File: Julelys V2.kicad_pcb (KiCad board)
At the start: 2 copper layers, 73 x 89 mm, 38 parts, among them J1 USB_B_Micro, J2 Conn_01x04_Pin, J3 Conn_01x14_Pin, SW1 SW_Push, SW2 SW_Push, U1 ESP32-C3-WROOM-02, U2 74HC4051, U3 AMS1117-3.3

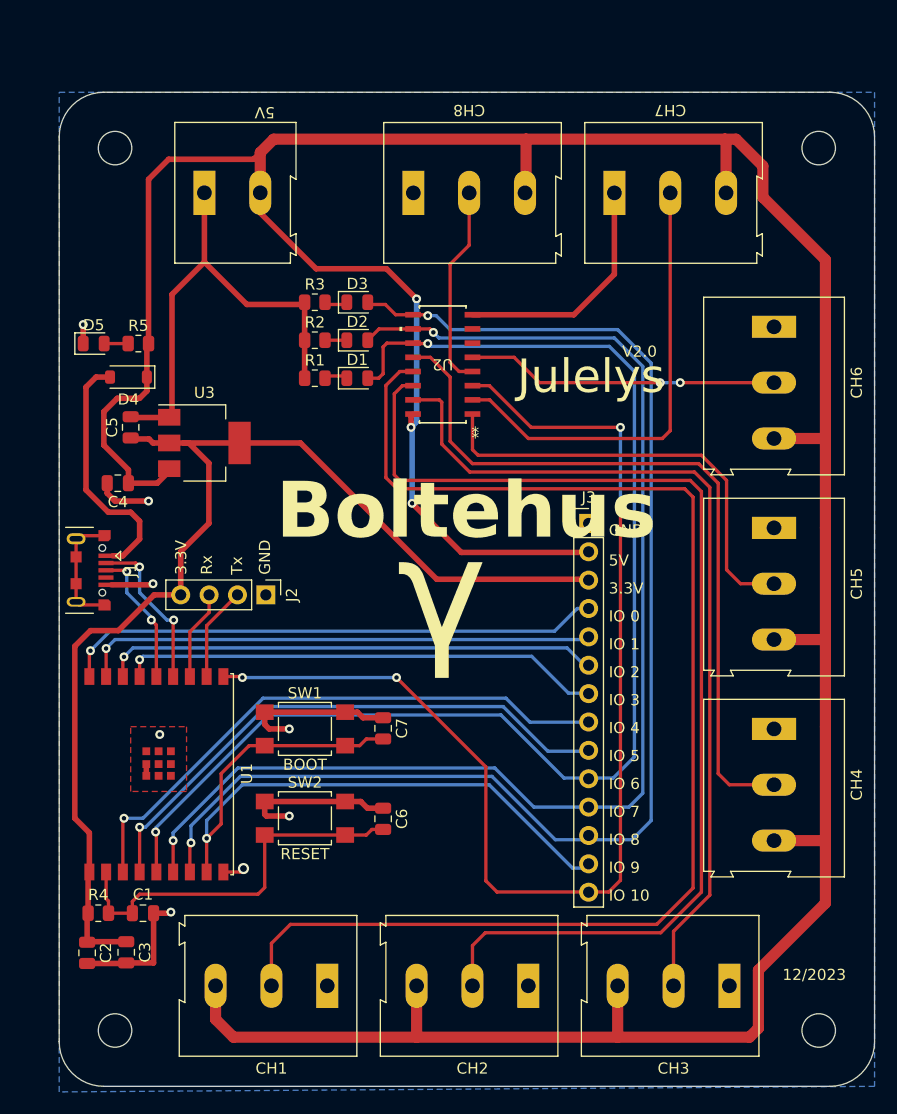
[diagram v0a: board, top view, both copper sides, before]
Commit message: version 3
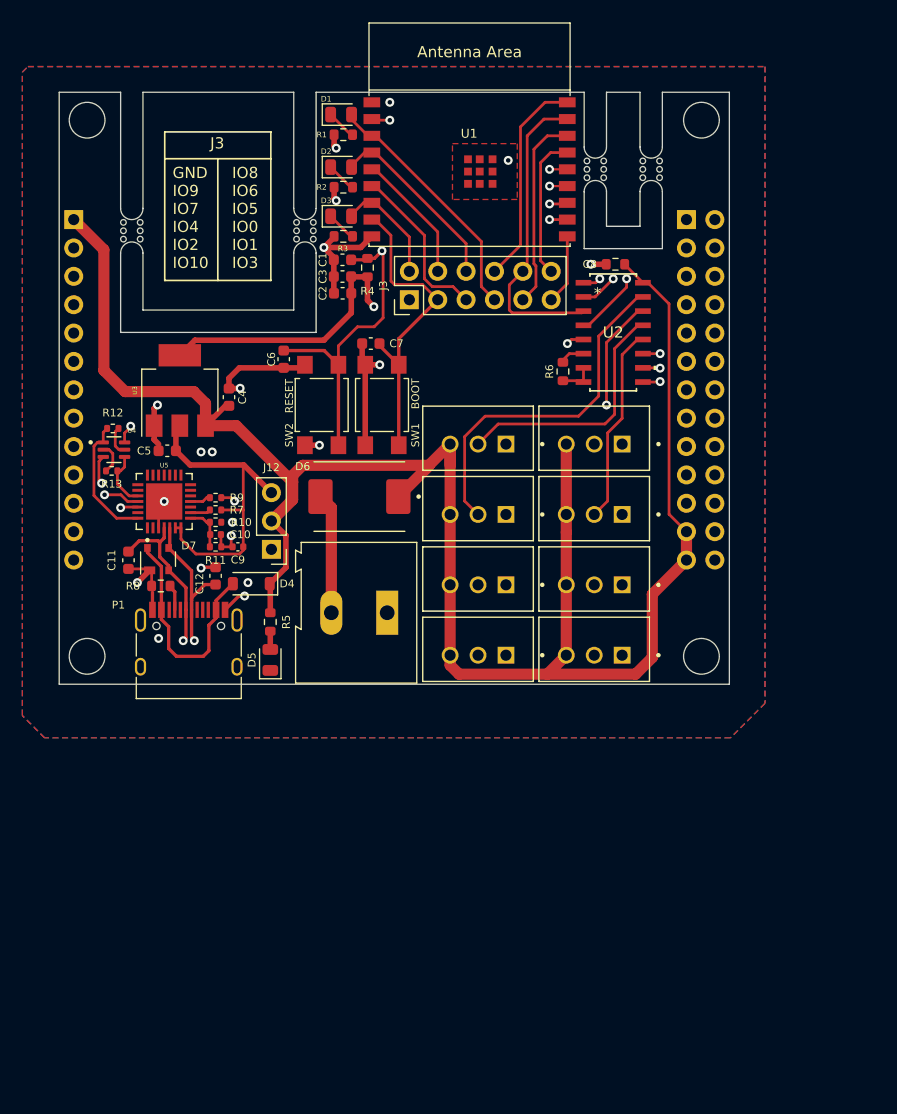
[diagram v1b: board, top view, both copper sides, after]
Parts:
- removed CH1, CH2, CH3, CH4, CH5, CH6, CH7, CH8: Screw_Terminal_01x03, TerminalBlock:TerminalBlock_Altech_AK300-3_P5.00mm
- added C10: 1uF/16V(10%), Capacitor_SMD:C_0402_1005Metric, F.Cu at (40.0, 54.6)
- added C11: 22pf, Capacitor_SMD:C_0603_1608Metric, F.Cu at (32.2, 56.9)
- added C12: 22pf, Capacitor_SMD:C_0603_1608Metric, F.Cu at (40.0, 58.3)
- added C8: 100nf, Resistor_SMD:R_0603_1608Metric, F.Cu at (75.8, 30.4)
- added C9: 10uF/25V(20%), Capacitor_SMD:C_0402_1005Metric, F.Cu at (42.0, 55.7)
- added D6: SS34-E3_57T, Diode_SMD:DIOM7959X262N, F.Cu at (52.9, 51.2)
- added D7: SP0503BAHT, Package_TO_SOT_SMD:SOT-143, F.Cu at (34.9, 56.8)
- added J10: B3B-XH-A, Connector:JST_B3B-XH-A, F.Cu at (63.5, 64.9)
- added J11: B3B-XH-A, Connector:JST_B3B-XH-A, F.Cu at (73.9, 64.9)
- added J12: Conn_01x03_Pin, Connector_PinHeader_2.54mm:PinHeader_1x03_P2.54mm_Vertical, F.Cu at (45.0, 55.9)
- added J4: B3B-XH-A, Connector:JST_B3B-XH-A, F.Cu at (63.5, 46.0)
- added J5: B3B-XH-A, Connector:JST_B3B-XH-A, F.Cu at (73.9, 46.0)
- added J6: B3B-XH-A, Connector:JST_B3B-XH-A, F.Cu at (63.5, 52.3)
- added J7: B3B-XH-A, Connector:JST_B3B-XH-A, F.Cu at (73.9, 52.3)
- added J8: B3B-XH-A, Connector:JST_B3B-XH-A, F.Cu at (63.5, 58.6)
- added J9: B3B-XH-A, Connector:JST_B3B-XH-A, F.Cu at (73.9, 58.6)
- added P1: USB_C_Plug_USB2.0, Connector_USB:USB_C_Receptacle_HRO_TYPE-C-31-M-12, F.Cu at (37.6, 65.4)
- added R10: 22.1K, Resistor_SMD:R_0402_1005Metric, F.Cu at (40.0, 53.5)
- added R11: 47.5K, Resistor_SMD:R_0402_1005Metric, F.Cu at (40.0, 55.7)
- added R12: 10k, Resistor_SMD:R_0402_1005Metric, F.Cu at (30.8, 45.1)
- added R13: 10k, Resistor_SMD:R_0402_1005Metric, F.Cu at (30.7, 48.9)
- added R6: 10K, Resistor_SMD:R_0603_1608Metric, F.Cu at (71.1, 40.0)
- added R7: 1K, Resistor_SMD:R_0402_1005Metric, F.Cu at (40.0, 52.4)
- added R8: 5.1K, Resistor_SMD:R_0603_1608Metric, F.Cu at (35.1, 59.2)
- added R9: 10K, Resistor_SMD:R_0402_1005Metric, F.Cu at (40.0, 51.3)
- added U4: BC847BDW1T1G, Transistor_Power_Module:SOT65P210X110-6N, F.Cu at (30.9, 47.0)
- added U5: CP2102N-A02-GQFN28, Connector_USB:QFN50P500X500X80-29N, F.Cu at (35.4, 51.6)
- added mouse-bite-2mm-slot: VAL**, footprints:mouse-bite-2mm-slot, F.Cu at (74.0, 21.9)
- added mouse-bite-2mm-slot: VAL**, footprints:mouse-bite-2mm-slot, F.Cu at (32.5, 27.4)
- added mouse-bite-2mm-slot: VAL**, footprints:mouse-bite-2mm-slot, F.Cu at (79.0, 21.9)
- added mouse-bite-2mm-slot: VAL**, footprints:mouse-bite-2mm-slot, F.Cu at (48.0, 27.4)
- C1, C2, C3, C4, C5, C6, C7: footprint Capacitor_SMD:C_0805_2012Metric -> Capacitor_SMD:C_0603_1608Metric
- H1, H2, H3, H4: footprint MountingHole:MountingHole_3mm -> MountingHole:MountingHole_3.2mm_M3
- J1: value USB_B_Micro -> Conn_02x13_Top_Bottom; footprint Connector_USB:USB_Micro-B_XKB_U254-051T-4BH83-F1S -> Connector_PinSocket_2.54mm:PinSocket_2x13_P2.54mm_Vertical; moved to B.Cu
- J2: value Conn_01x04_Pin -> Conn_01x13; footprint Connector_PinHeader_2.54mm:PinHeader_1x04_P2.54mm_Vertical -> Connector_PinSocket_2.54mm:PinSocket_1x13_P2.54mm_Vertical; moved to B.Cu
- J3: value Conn_01x14_Pin -> Conn_02x06_Odd_Even; footprint Connector_PinHeader_2.54mm:PinHeader_1x14_P2.54mm_Vertical -> Connector_PinHeader_2.54mm:PinHeader_2x06_P2.54mm_Vertical
- R1, R2, R3, R4, R5: footprint Resistor_SMD:R_0805_2012Metric -> Resistor_SMD:R_0603_1608Metric
- moved C3 63.5 mm to (51.4, 31.5), turned to 180 degrees
- moved C2 63.3 mm to (51.4, 33.0), turned to 180 degrees
- moved J1 62.7 mm to (82.2, 26.4), turned to 180 degrees
- moved R4 62.6 mm to (53.6, 30.7), turned to 90 degrees
- moved C1 61.2 mm to (51.4, 30.0), turned to 180 degrees
- moved U1 61.1 mm to (62.7, 21.8), turned to 0 degrees
- moved C6 42.1 mm to (46.1, 38.9), turned to 90 degrees
- moved V_IN1 41.0 mm to (55.4, 61.6), turned to 180 degrees
- moved J2 37.7 mm to (27.3, 26.4), turned to 180 degrees
- moved SW2 37.0 mm to (49.5, 43.0), turned to 90 degrees
- moved H4 35.1 mm to (83.5, 65.5)
- moved C7 34.5 mm to (53.9, 37.5), turned to 0 degrees
- moved H3 33.6 mm to (28.5, 65.5)
- moved D5 32.4 mm to (44.9, 65.8), turned to 90 degrees
- moved SW1 29.8 mm to (54.9, 43.0), turned to 90 degrees
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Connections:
- D4 pad 2: Net-(D4-A) -> VBUS
- J1 pad 1: Net-(D4-A) -> unconnected-(J1-Pin_1-Pad1)
- J1 pad 2: USB_D- -> GND
- J1 pad 3: USB_D+ -> CS
- J1 pad 4: unconnected-(J1-ID-Pad4) -> CLK
- J1 pad 5: GND -> unconnected-(J1-Pin_5-Pad5)
- J1 pad 6: unconnected-(J1-Shield-Pad6) -> IO2
- J2 pad 1: GND -> +5V
- J2 pad 2: U-RX -> GND
- J2 pad 3: U-TX -> unconnected-(J2-Pin_3-Pad3)
- J2 pad 4: +3.3V -> unconnected-(J2-Pin_4-Pad4)
- J3 pad 10: A0 -> IO1
- J3 pad 11: A1 -> CS
- J3 pad 12: A2 -> IO3
- J3 pad 2: +5V -> A2
- J3 pad 3: +3.3V -> IO9
- J3 pad 4: IO0 -> CLK
- J3 pad 5: IO1 -> IO7
- J3 pad 6: IO2 -> A1
- J3 pad 7: IO3 -> A0
- J3 pad 8: IO4 -> IO0
- J3 pad 9: IO5 -> IO2
- U1 pad 10: IO10 -> CS
- U1 pad 11: U-RX -> RXD
- U1 pad 12: U-TX -> TXD
- U1 pad 3: IO4 -> A0
- U1 pad 4: IO5 -> A1
- U1 pad 5: A0 -> CLK
- U1 pad 6: A1 -> IO7
- U2 pad 3: IO10 -> IO1
- U2 pad 6: unconnected-(U2-~{E}-Pad6) -> Net-(U2-~{E})
- U2 pad 7: unconnected-(U2-VEE-Pad7) -> GND
- V_IN1 pad 2: +5V -> Net-(V_IN1-Pin_2)
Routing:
- net +5V: track 319.8 -> 174.2 mm, vias 3 -> 0
- net IO10: track 105.3 -> 0.00 mm, vias 4 -> 0
- net Net-(U2-A0): track 118.0 -> 22.6 mm
- net Net-(U2-A1): track 99.3 -> 14.0 mm, vias 0 -> 1
- net A2: track 118.8 -> 43.7 mm, vias 2 -> 1
- net USB_D+: track 11.9 -> 85.8 mm, vias 2 -> 3
- net USB_D-: track 14.1 -> 83.6 mm, vias 2 -> 3
- net A1: track 114.6 -> 47.6 mm, vias 2 -> 1
- net A0: track 116.3 -> 50.7 mm, vias 2 -> 1
- net TXD: track 0.00 -> 62.0 mm, vias 0 -> 2
- net RXD: track 0.00 -> 58.7 mm, vias 0 -> 2
- net GND: track 117.8 -> 62.0 mm, vias 8 -> 16
- net IO4: track 51.9 -> 0.00 mm, vias 1 -> 0
- net IO5: track 50.5 -> 0.00 mm, vias 1 -> 0
- net Net-(U2-A3): track 66.8 -> 17.8 mm
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- added copper zone on In1.Cu, net GND
- added copper zone on In2.Cu, net GND
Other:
- board size 73 x 89 mm -> 60 x 53 mm
- copper layers 2 -> 4
- board text added: "02/2025"
- board text added: "GND IO9 IO7 IO4 IO2 IO10"
- board text added: "IO8 IO6 IO5 IO0 IO1 IO3"
- board text added: "J3"
- board text added: "V3.0"
- board text added: "∑"
- board text removed: "12/2023"
- board text removed: "IO 0"
- board text removed: "IO 1"
- board text removed: "IO 10"
- board text removed: "IO 2"
- board text removed: "IO 3"
- board text removed: "IO 4"
- board text removed: "IO 5"
- board text removed: "IO 6"
- board text removed: "IO 7"
- board text removed: "IO 8"
- board text removed: "IO 9"
- board text removed: "Rx"
- board text removed: "Tx"
- board text removed: "V2.0"
- board text removed: "γ"
